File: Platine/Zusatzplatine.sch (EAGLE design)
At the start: 31 parts, among them X2 22-23-2081, X3 22-23-2081, X4 22-23-2101

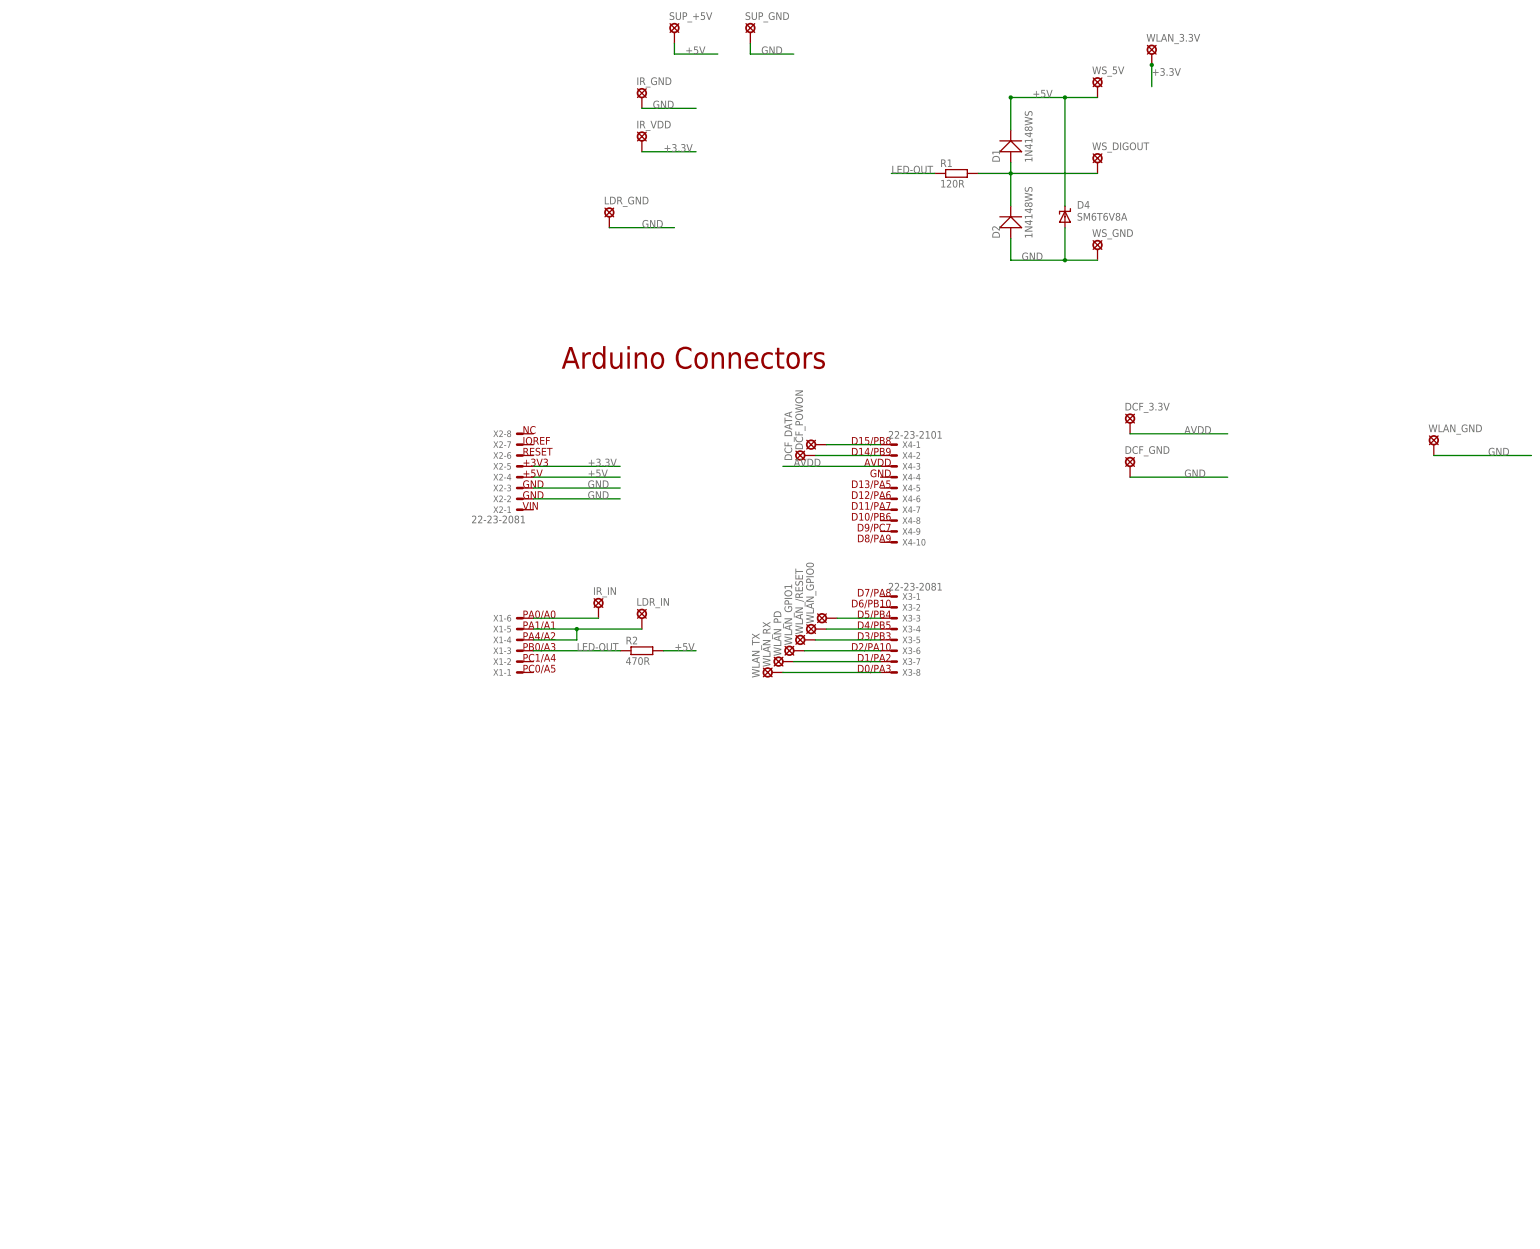
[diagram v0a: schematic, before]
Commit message: Reworked Board Design
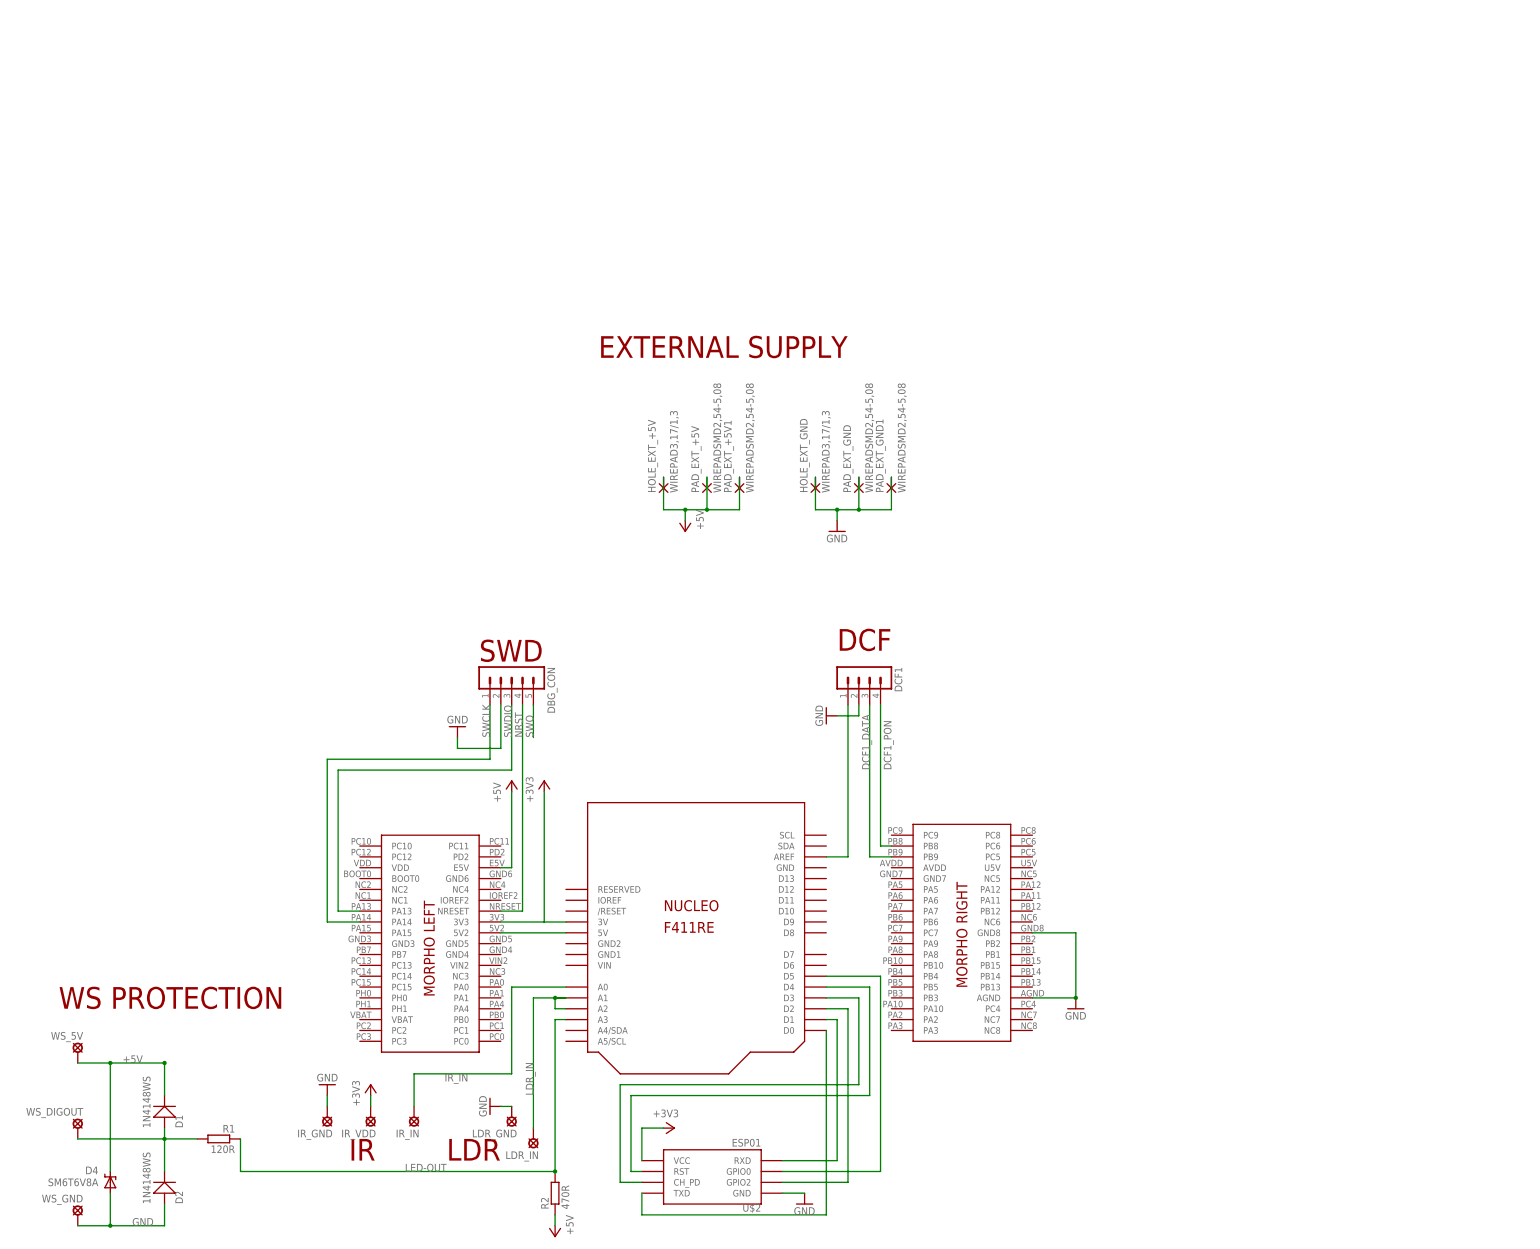
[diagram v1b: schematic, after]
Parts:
- removed DCF_3.3V, DCF_DATA, DCF_GND, DCF_POWON, SUP_+5V, SUP_GND, WLAN_/RESET, WLAN_3.3V, WLAN_GND, WLAN_GPIO0, WLAN_GPIO1, WLAN_PD, WLAN_RX, WLAN_TX: SE14, solpad:SE14
- removed X1: (no value), con-molex:22-23-2061
- removed X2, X3: 22-23-2081, con-molex:22-23-2081
- removed X4: 22-23-2101, con-molex:22-23-2101
- added DBG_CON: (no value), con-lstb:MA05-1
- added DCF1: (no value), con-lstb:MA04-1
- added HOLE_EXT_+5V, HOLE_EXT_GND: WIREPAD3,17/1,3, wirepad:WIREPAD3,17/1,3
- added PAD_EXT_+5V, PAD_EXT_+5V1, PAD_EXT_GND, PAD_EXT_GND1: WIREPADSMD2,54-5,08, wirepad:WIREPADSMD2,54-5,08
- added U$1: NUCLEO_F411RE, Stm32nucleo:NUCLEO_F411RE
- added U$2: ESP01, esp8266modules:ESP01
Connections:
- removed net +3.3V: IR_VDD.MP, WLAN_3.3V.MP, X2-5.S
- removed net AVDD: DCF_3.3V.MP, X4-3.S
- removed net N$10: DCF_POWON.MP, X4-1.S
- removed net N$11: DCF_DATA.MP, X4-2.S
- removed net N$3: LDR_IN.MP, X1-4.S, X1-5.S
- removed net N$4: WLAN_RX.MP, X3-7.S
- removed net N$5: WLAN_PD.MP, X3-6.S
- removed net N$6: WLAN_GPIO1.MP, X3-5.S
- removed net N$7: WLAN_/RESET.MP, X3-4.S
- removed net N$9: WLAN_GPIO0.MP, X3-3.S
- new net +3V3: IR_VDD.MP, U$1.3V, U$1.3V3, U$2.VCC
- new net DCF1_DATA: DCF1.3, U$1.PB9
- new net DCF1_PON: DCF1.4, U$1.PB8
- new net IR_IN: IR_IN.MP, U$1.A0
- new net LDR_IN: LDR_IN.MP, U$1.A1, U$1.A2
- new net N$12: U$1.D5, U$2.GPIO0
- new net N$13: U$1.D4, U$2.RST
- new net N$14: U$1.D3, U$2.CH_PD
- new net N$15: U$1.D0, U$2.TXD
- new net N$16: U$1.D1, U$2.RXD
- new net N$17: U$1.D2, U$2.GPIO2
- new net NRST: DBG_CON.4, U$1.NRESET
- new net SWCLK: DBG_CON.1, U$1.PA14
- new net SWDIO: DBG_CON.3, U$1.PA13
- new net SWO: DBG_CON.5
- net +5V: now also HOLE_EXT_+5V.P, PAD_EXT_+5V.P, PAD_EXT_+5V1.P, R2.1, U$1.E5V; no longer R2.2, SUP_+5V.MP, X2-4.S
- net GND: now also DBG_CON.2, DCF1.2, HOLE_EXT_GND.P, PAD_EXT_GND.P, PAD_EXT_GND1.P, U$1.AGND, U$1.GND8, U$2.GND; no longer DCF_GND.MP, SUP_GND.MP, X2-2.S, X2-3.S
- net LED-OUT: now also R2.2, U$1.A3; no longer R2.1, X1-3.S
- net N$1: now also DCF1.1, U$1.AREF; no longer WLAN_TX.MP, X3-8.S
- net N$2: now also U$1.5V, U$1.5V2; no longer IR_IN.MP, X1-6.S
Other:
- note added: "DCF"
- note added: "EXTERNAL SUPPLY"
- note added: "IR"
- note added: "LDR"
- note added: "SWD"
- note added: "WS PROTECTION"
- note removed: "+3V3"
- note removed: "+5V"
- note removed: "AVDD"
- note removed: "Arduino Connectors"
- note removed: "D0/PA3"
- note removed: "D1/PA2"
- note removed: "D10/PB6"
- note removed: "D11/PA7"
- note removed: "D12/PA6"
- note removed: "D13/PA5"
- note removed: "D14/PB9"
- note removed: "D15/PB8"
- note removed: "D2/PA10"
- note removed: "D3/PB3"
- note removed: "D4/PB5"
- note removed: "D5/PB4"
- note removed: "D6/PB10"
- note removed: "D7/PA8"
- note removed: "D8/PA9"
- note removed: "D9/PC7"
- note removed: "GND"
- note removed: "IOREF"
- note removed: "NC"
- note removed: "PA0/A0"
- note removed: "PA1/A1"
- note removed: "PA4/A2"
- note removed: "PB0/A3"
- note removed: "PC0/A5"
- note removed: "PC1/A4"
- note removed: "RESET"
- note removed: "VIN"
- moved on the sheet: D1, D2, D4, IR_GND, IR_IN, IR_VDD, LDR_GND, LDR_IN, R1, R2, WS_5V, WS_DIGOUT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
